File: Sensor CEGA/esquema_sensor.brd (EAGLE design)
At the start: 69.8 x 73.3 mm, 8 parts, among them J1 DCJ0202

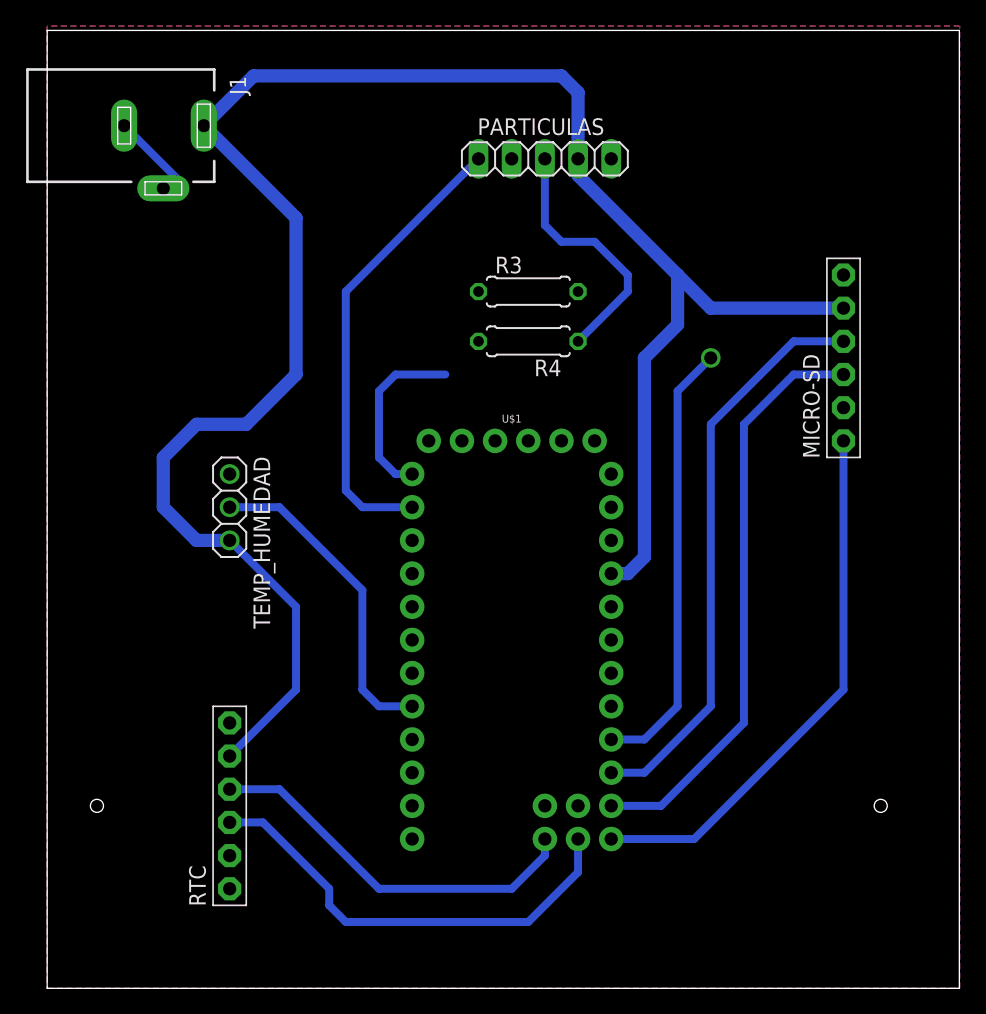
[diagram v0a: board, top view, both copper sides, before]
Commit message: last version and fotos
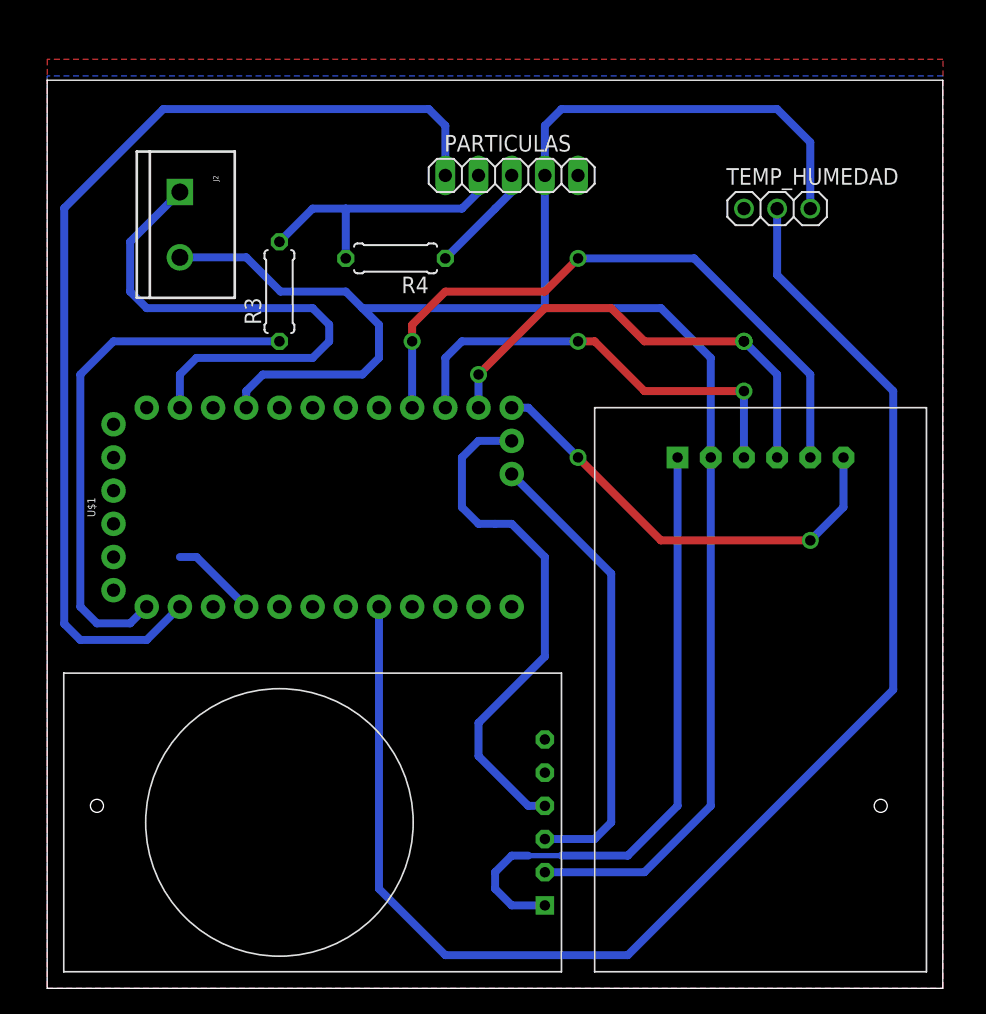
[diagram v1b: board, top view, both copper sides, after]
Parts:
- removed J1: DCJ0202, con-jack:DCJ0202
- removed MICRO-SD: (no value), adafruit:1X06-BIG
- added J2: (no value), SparkFun-Connectors:SCREWTERMINAL-5MM-2
- added SD_READER: MICRO_SD_READER, fablab_uchile:MICRO_SD_READER
- R3: value (none) -> 100
- R4: value (none) -> 200
- RTC: value (none) -> DS3231_RTC; device adafruit:1X06-BIG -> fablab_uchile:DS3231_RTC
- U$1: value PRO_MINI_CEGA -> PRO_MINI_CEGAPRO_MINI_MOD; device fablab_uchile:ARDUINO_PRO_MINI -> fablab_uchile:ARDUINO_PRO_MINI_MOD
- moved TEMP_HUMEDAD 47.7 mm to (55.9, 59.7), turned to 0 degrees
- moved R3 19.0 mm to (17.8, 53.3), turned to 90 degrees
- moved U$1 18.3 mm to (20.3, 36.8), turned to 90 degrees
- moved RTC 14.0 mm to (27.9, 12.7), turned to 270 degrees
- moved R4 12.0 mm to (26.7, 55.9)
- moved PARTICULAS 2.84 mm to (35.6, 62.2)
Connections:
- net N$5 renamed D1
- net N$6 renamed D0
- net N$8 renamed D5
- removed net GNDA: J1.2, J1.3, MICRO-SD.6, PARTICULAS.3, R4.1, RTC.6, TEMP_HUMEDAD.1, U$1.23, U$1.4
- removed net N$10: MICRO-SD.4, U$1.15
- removed net N$11: MICRO-SD.3, U$1.14
- removed net N$12: MICRO-SD.2, U$1.16
- removed net N$13: MICRO-SD.1, U$1.13
- new net D10: SD_READER.CS, U$1.13
- new net D11: SD_READER.MOSI, U$1.14
- new net D12: SD_READER.MISO, U$1.15
- new net D13: SD_READER.SCK, U$1.16
- new net GND: J2.1, PARTICULAS.3, R4.1, RTC.GND, SD_READER.GND, TEMP_HUMEDAD.1, U$1.23, U$1.4
- net +5V: now also J2.2, RTC.VCC, SD_READER.VCC; no longer J1.1, MICRO-SD.5, RTC.5
- net A4: now also RTC.SDA; no longer RTC.4
- net A5: now also RTC.SCL; no longer RTC.3
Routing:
- net GND: track 0.00 -> 104.6 mm
- net D5: track 24.7 -> 112.0 mm
- net D13: track 0.00 -> 49.0 mm, vias 0 -> 2
- net N$11: track 44.8 -> 0.00 mm
- net N$10: track 44.1 -> 0.00 mm
- net D1: track 35.2 -> 78.9 mm
- net N$13: track 41.6 -> 0.00 mm
- net D11: track 0.00 -> 36.0 mm, vias 0 -> 3
- net D10: track 0.00 -> 34.5 mm, vias 0 -> 2
- net N$12: track 33.9 -> 0.00 mm, vias 1 -> 0
- net D12: track 0.00 -> 33.9 mm, vias 0 -> 2
- net GNDA: track 26.8 -> 0.00 mm
- net D0: track 13.8 -> 40.2 mm
- net N$2: track 0.00 -> 21.9 mm
- net +5V: track 161.7 -> 150.7 mm
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- added copper zone on layer 1, net GND
- added copper zone on layer 16, net GND
- removed copper zone on layer 1, net GNDA
- removed copper zone on layer 16, net GNDA
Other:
- board size 69.8 x 73.3 mm -> 68.6 x 69.5 mm
